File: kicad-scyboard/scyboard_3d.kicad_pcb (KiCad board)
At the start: 2 copper layers, 144 x 96.5 mm, 48 parts

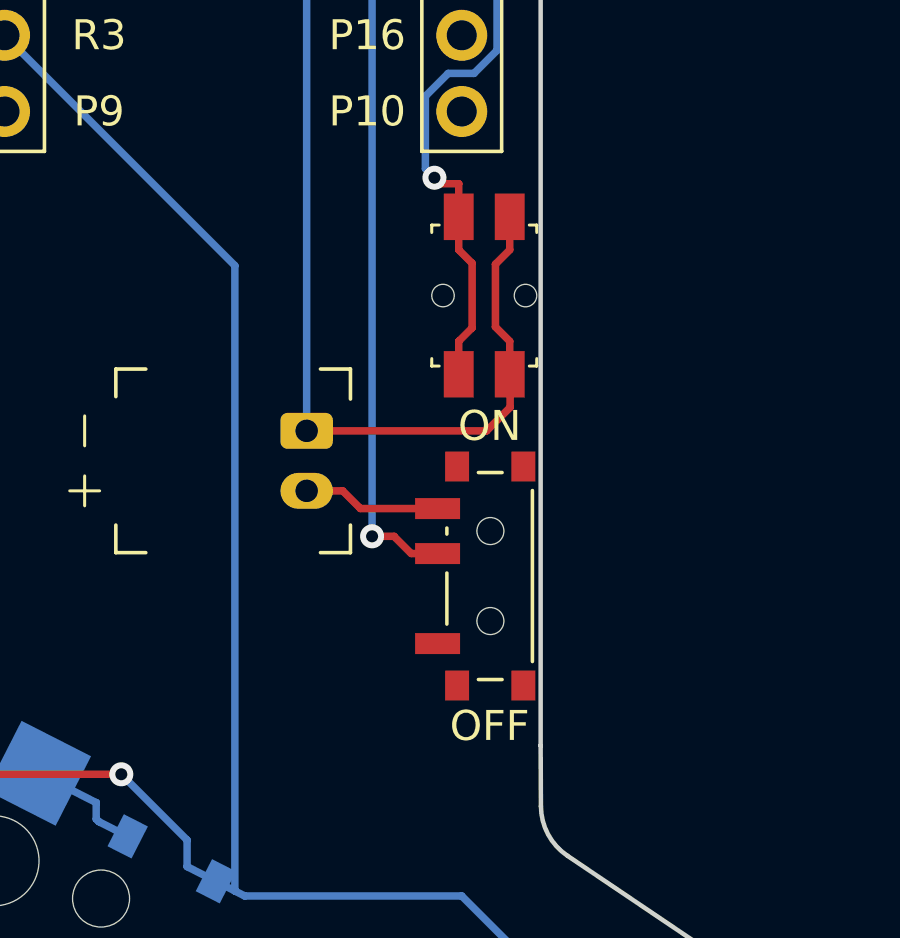
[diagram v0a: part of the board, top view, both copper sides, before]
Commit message: Compile
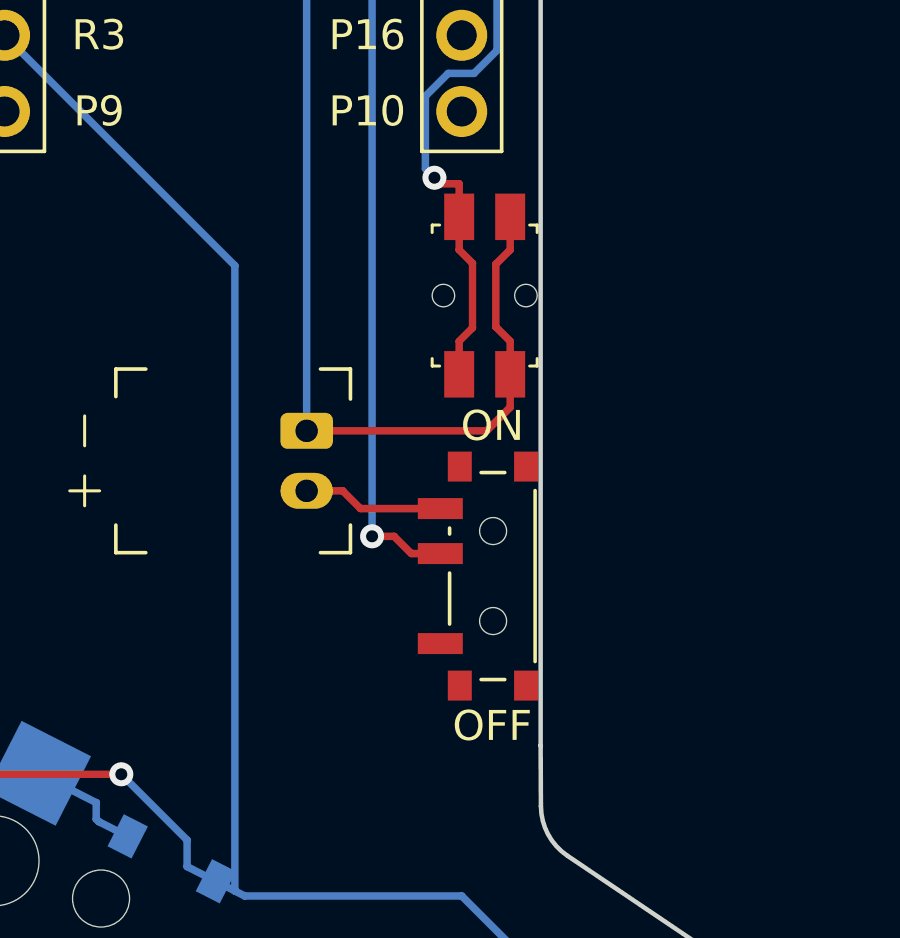
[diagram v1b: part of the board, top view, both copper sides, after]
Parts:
- D1, D10, D11, D12, D13, D14, D15, D16, D17, D18, D19, D2, D20, D21, D22, D3, D4, D5, D6, D7, D8, D9: footprint ceoloide:diode_tht_sod123 -> custom:custom_diode_tht_sod123
- S1, S10, S11, S12, S13, S14, S15, S16, S17, S18, S19, S2, S20, S21, S3, S4, S5, S6, S7, S8, S9: footprint ceoloide:switch_choc_v1_v2 -> custom:custom_switch_choc_v1_v2
- S22: footprint ceoloide:switch_choc_v1_v2 -> custom:custom_switch_choc_v1_v2_1.5u
- moved PWR1 0.09 mm to (168.1, 92.9)
